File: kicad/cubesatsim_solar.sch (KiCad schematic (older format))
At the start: 23 parts, among them J1 Sensor Inputs, J10 INA219 Sensor Board, J11 INA219 Sensor Board, J12 INA219 Sensor Board, J13 3.5mm TRS Audio Jack with 2 S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, J14 RBF connector, J2 Battery In/Out, J3 Vout to MoPOWER, J4 Vdc In, J5 RBF Switch, J6 Expansion Interface, J7 INA219 Sensor Board, J8 INA219 Sensor Board, J9 INA219 Sensor Board, P3 Raspberry Pi GPIO Connector, U1 Variable Boost Converter Modu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

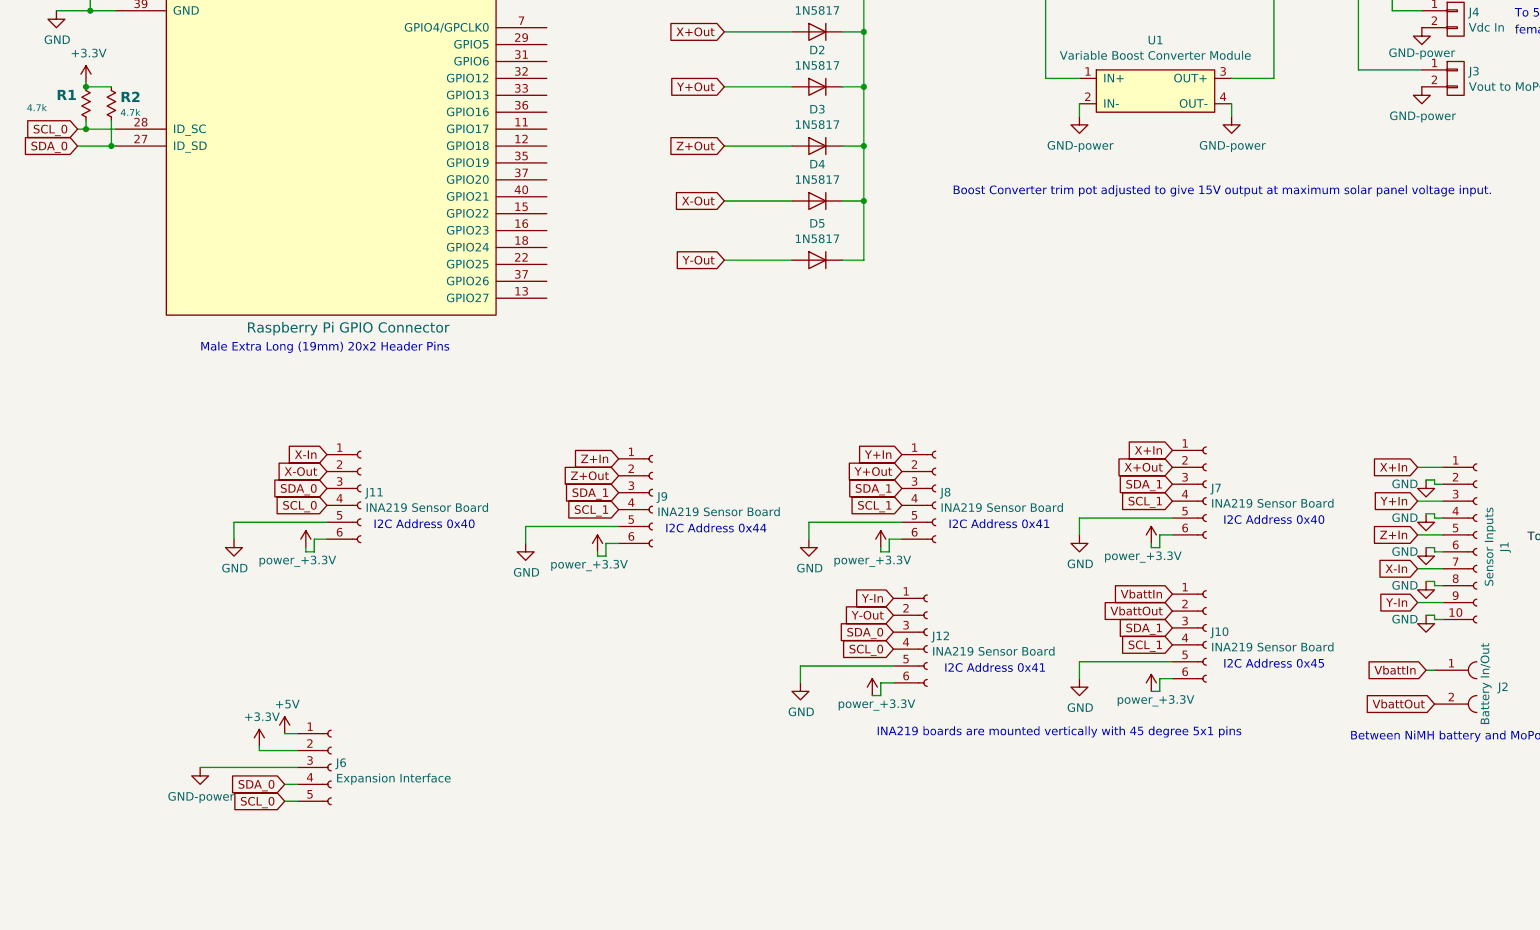
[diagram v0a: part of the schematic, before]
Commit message: Preliminary PCB Design
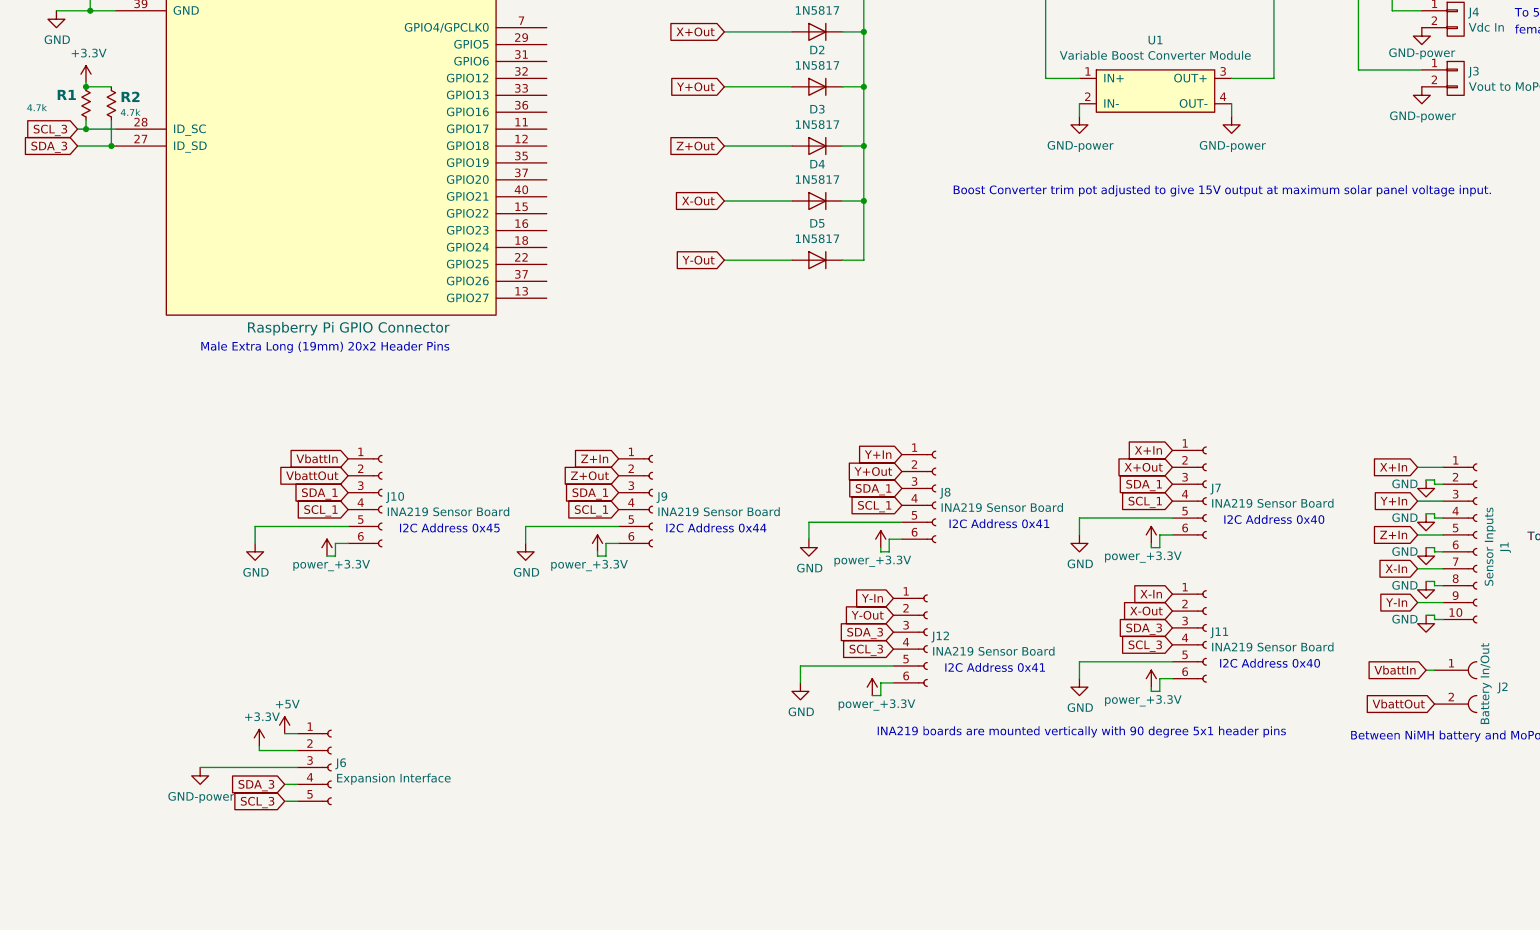
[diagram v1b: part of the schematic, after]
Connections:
- net SCL_0 renamed SCL_3
- net SDA_0 renamed SDA_3
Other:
- note added: "INA219 boards are mounted vertically with 90 degree 5x1 header pins"
- note removed: "INA219 boards are mounted vertically with 45 degree 5x1 pins"
- moved on the sheet: J10, J11
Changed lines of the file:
@@
 Sheet 1 1
 Title "AMSAT CubeSat Simulator Solar Panel Board"
-Date "December 8, 2018"
-Rev "Beta1"
+Date "December 13, 2018"
+Rev "Beta1.1"
 Comp "See https://github.com/alanbjohnston/cubesatsim"
 Comment1 ""
@@
 	7325 5475 7325 5450
 Text GLabel 975  3100 0    50   Input ~ 0
-SDA_0
+SDA_3
 Text GLabel 975  3000 0    50   Input ~ 0
-SCL_0
+SCL_3
 $Comp
 L pihat_template-rescue:Raspberry_Pi_+_Conn-pihat_template-rescue P3
@@
 Wire Wire Line
 	1025 3000 1200 3000
-Text GLabel 7450 5750 0    50   Input ~ 0
+Text GLabel 2575 4950 0    50   Input ~ 0
 VbattIn
-Text GLabel 7450 5850 0    50   Input ~ 0
+Text GLabel 2575 5050 0    50   Input ~ 0
 VbattOut
-Text GLabel 7450 5950 0    50   Input ~ 0
+Text GLabel 2575 5150 0    50   Input ~ 0
 SDA_1
-Text GLabel 7450 6050 0    50   Input ~ 0
+Text GLabel 2575 5250 0    50   Input ~ 0
 SCL_1
 $Comp
 L pihat_template-rescue:GND-power #PWR05
 U 1 1 5BF9E33A
-P 6900 6250
-F 0 "#PWR05" H 6900 6000 50  0001 C CNN
-F 1 "GND" H 6905 6077 50  0000 C CNN
-F 2 "" H 6900 6250 50  0001 C CNN
-F 3 "" H 6900 6250 50  0001 C CNN
-	1    6900 6250
-	1    0    0    -1
-$EndComp
-Wire Wire Line
-	6900 6250 6900 6150
-Wire Wire Line
-	6900 6150 7450 6150
+P 2025 5450
+F 0 "#PWR05" H 2025 5200 50  0001 C CNN
+F 1 "GND" H 2030 5277 50  0000 C CNN
+F 2 "" H 2025 5450 50  0001 C CNN
+F 3 "" H 2025 5450 50  0001 C CNN
+	1    2025 5450
+	1    0    0    -1
+$EndComp
+Wire Wire Line
+	2025 5450 2025 5350
+Wire Wire Line
+	2025 5350 2575 5350
 $Comp
 L pihat_template-rescue:Conn_01x06_Female-Connector J10
 U 1 1 5BF9E342
-P 7650 5950
-F 0 "J10" H 7678 5926 50  0000 L CNN
-F 1 "INA219 Sensor Board" H 7678 5835 50  0000 L CNN
-F 2 "Connector_PinHeader_2.54mm:PinHeader_1x06_P2.54mm_Vertical" H 7650 5950 50  0001 C CNN
-F 3 "~" H 7650 5950 50  0001 C CNN
-	1    7650 5950
-	1    0    0    -1
-$EndComp
-Wire Wire Line
-	7450 6250 7375 6250
-Wire Wire Line
-	7375 6250 7375 6325
-Wire Wire Line
-	7375 6325 7325 6325
+P 2775 5150
+F 0 "J10" H 2803 5126 50  0000 L CNN
+F 1 "INA219 Sensor Board" H 2803 5035 50  0000 L CNN
+F 2 "Connector_PinHeader_2.54mm:PinHeader_1x06_P2.54mm_Vertical" H 2775 5150 50  0001 C CNN
+F 3 "~" H 2775 5150 50  0001 C CNN
+	1    2775 5150
+	1    0    0    -1
+$EndComp
+Wire Wire Line
+	2575 5450 2500 5450
+Wire Wire Line
+	2500 5450 2500 5525
+Wire Wire Line
+	2500 5525 2450 5525
 $Comp
 L pihat_template-rescue:+3.3V-PiHatAx5043-cache #PWR0101
@@
 $EndComp
 Text GLabel 2200 6875 0    50   Input ~ 0
-SDA_0
+SDA_3
 Text GLabel 2200 6975 0    50   Input ~ 0
-SCL_0
+SCL_3
 Wire Wire Line
 	2275 6875 2200 6875
@@
 L pihat_template-rescue:power_+3.3V-PiHatAx5043-cache #PWR0115
 U 1 1 5BFB928B
-P 7325 6325
-F 0 "#PWR0115" H 7325 6175 50  0001 C CNN
-F 1 "power_+3.3V" H 7350 6275 50  0000 C CNN
-F 2 "" H 7325 6325 50  0001 C CNN
-F 3 "" H 7325 6325 50  0001 C CNN
-	1    7325 6325
+P 2450 5525
+F 0 "#PWR0115" H 2450 5375 50  0001 C CNN
+F 1 "power_+3.3V" H 2475 5475 50  0000 C CNN
+F 2 "" H 2450 5525 50  0001 C CNN
+F 3 "" H 2450 5525 50  0001 C CNN
+	1    2450 5525
 	1    0    0    -1
 $EndComp
 Text Notes 7750 5350 0    50   ~ 0
 I2C Address 0x40
-Text Notes 7750 6200 0    50   ~ 0
+Text Notes 2875 5400 0    50   ~ 0
 I2C Address 0x45
 Text GLabel 5850 4925 0    50   Input ~ 0
@@
 Text Notes 4450 5400 0    50   ~ 0
 I2C Address 0x44\n
-Text GLabel 2450 4925 0    50   Input ~ 0
+Text GLabel 7450 5750 0    50   Input ~ 0
 X-In
-Text GLabel 2450 5025 0    50   Input ~ 0
+Text GLabel 7450 5850 0    50   Input ~ 0
 X-Out
-Text GLabel 2450 5125 0    50   Input ~ 0
-SDA_0
-Text GLabel 2450 5225 0    50   Input ~ 0
-SCL_0
+Text GLabel 7450 5950 0    50   Input ~ 0
+SDA_3
+Text GLabel 7450 6050 0    50   Input ~ 0
+SCL_3
 $Comp
 L pihat_template-rescue:GND-power #PWR0120
 U 1 1 5BFBED52
-P 1900 5425
-F 0 "#PWR0120" H 1900 5175 50  0001 C CNN
-F 1 "GND" H 1905 5252 50  0000 C CNN
-F 2 "" H 1900 5425 50  0001 C CNN
-F 3 "" H 1900 5425 50  0001 C CNN
-	1    1900 5425
-	1    0    0    -1
-$EndComp
-Wire Wire Line
-	1900 5425 1900 5325
-Wire Wire Line
-	1900 5325 2450 5325
+P 6900 6250
+F 0 "#PWR0120" H 6900 6000 50  0001 C CNN
+F 1 "GND" H 6905 6077 50  0000 C CNN
+F 2 "" H 6900 6250 50  0001 C CNN
+F 3 "" H 6900 6250 50  0001 C CNN
+	1    6900 6250
+	1    0    0    -1
+$EndComp
+Wire Wire Line
+	6900 6250 6900 6150
+Wire Wire Line
+	6900 6150 7450 6150
 $Comp
 L pihat_template-rescue:Conn_01x06_Female-Connector J11
 U 1 1 5BFBED5A
-P 2650 5125
-F 0 "J11" H 2678 5101 50  0000 L CNN
-F 1 "INA219 Sensor Board" H 2678 5010 50  0000 L CNN
-F 2 "Connector_PinHeader_2.54mm:PinHeader_1x06_P2.54mm_Vertical" H 2650 5125 50  0001 C CNN
-F 3 "~" H 2650 5125 50  0001 C CNN
-	1    2650 5125
-	1    0    0    -1
-$EndComp
-Wire Wire Line
-	2450 5425 2375 5425
-Wire Wire Line
-	2375 5425 2375 5500
-Wire Wire Line
-	2375 5500 2325 5500
-Wire Wire Line
-	2325 5500 2325 5475
+P 7650 5950
+F 0 "J11" H 7678 5926 50  0000 L CNN
+F 1 "INA219 Sensor Board" H 7678 5835 50  0000 L CNN
+F 2 "Connector_PinHeader_2.54mm:PinHeader_1x06_P2.54mm_Vertical" H 7650 5950 50  0001 C CNN
+F 3 "~" H 7650 5950 50  0001 C CNN
+	1    7650 5950
+	1    0    0    -1
+$EndComp
+Wire Wire Line
+	7450 6250 7375 6250
+Wire Wire Line
+	7375 6250 7375 6325
+Wire Wire Line
+	7375 6325 7325 6325
+Wire Wire Line
+	7325 6325 7325 6300
 $Comp
 L pihat_template-rescue:power_+3.3V-PiHatAx5043-cache #PWR0121
 U 1 1 5BFBED64
-P 2325 5475
-F 0 "#PWR0121" H 2325 5325 50  0001 C CNN
-F 1 "power_+3.3V" H 2275 5400 50  0000 C CNN
-F 2 "" H 2325 5475 50  0001 C CNN
-F 3 "" H 2325 5475 50  0001 C CNN
-	1    2325 5475
-	1    0    0    -1
-$EndComp
-Text Notes 2725 5375 0    50   ~ 0
+P 7325 6300
+F 0 "#PWR0121" H 7325 6150 50  0001 C CNN
+F 1 "power_+3.3V" H 7275 6225 50  0000 C CNN
+F 2 "" H 7325 6300 50  0001 C CNN
+F 3 "" H 7325 6300 50  0001 C CNN
+	1    7325 6300
+	1    0    0    -1
+$EndComp
+Text Notes 7725 6200 0    50   ~ 0
 I2C Address 0x40
 Text GLabel 5800 5775 0    50   Input ~ 0
@@
 Y-Out
 Text GLabel 5800 5975 0    50   Input ~ 0
-SDA_0
+SDA_3
 Text GLabel 5800 6075 0    50   Input ~ 0
-SCL_0
+SCL_3
 $Comp
 L pihat_template-rescue:GND-power #PWR0122
@@
 Between NiMH battery and MoPower Board
 Text Notes 5700 6600 0    50   ~ 0
-INA219 boards are mounted vertically with 45 degree 5x1 pins
+INA219 boards are mounted vertically with 90 degree 5x1 header pins
 Text Notes 1700 4325 0    50   ~ 0
 Male Extra Long (19mm) 20x2 Header Pins
